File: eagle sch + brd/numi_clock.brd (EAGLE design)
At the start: 100 x 80 mm, 35 parts, among them IC1 MEGA8-AI, IC2 LM75, Q1 12MHz, Y1 32.768kHz

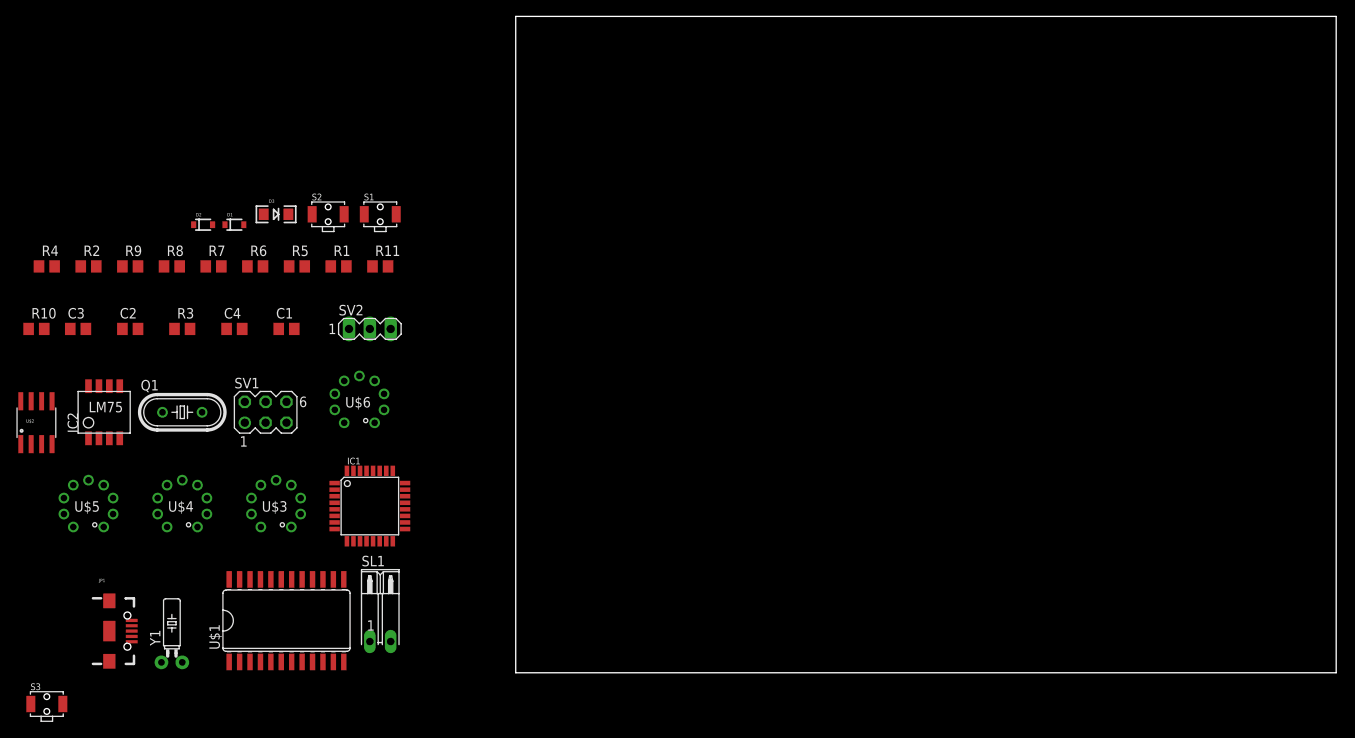
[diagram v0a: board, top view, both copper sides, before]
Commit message: minor changes
minor changes
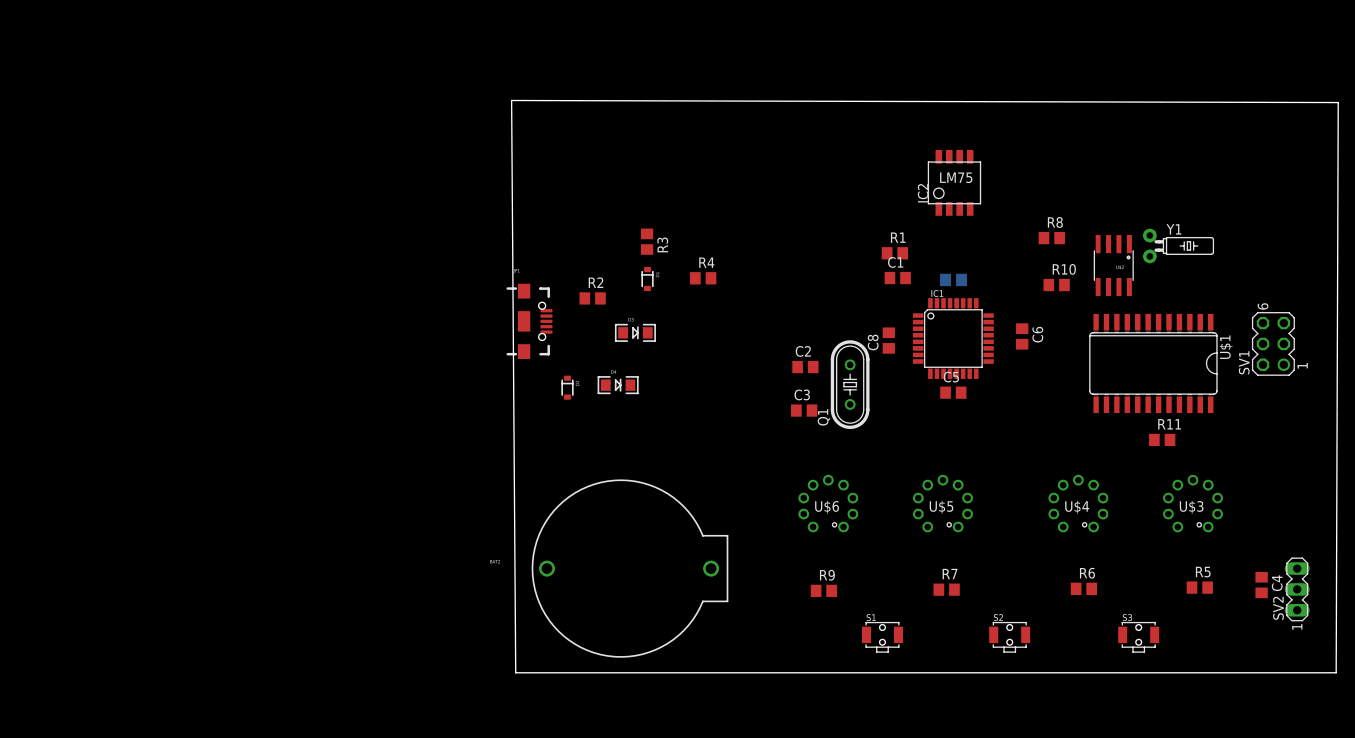
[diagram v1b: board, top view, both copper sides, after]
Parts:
- removed SL1: VBATT, con-amp-quick:02PA
- added BAT2: cr2032, SparkFun:BATTCOM_20MM_PTH
- added C5, C6, C7, C8: 100nF, rcl:C0805
- added D4: red, SparkFun-LED:LED-1206
- moved S3 133.3 mm to (75.9, 4.62)
- moved U$2 132.7 mm to (72.9, 49.6), turned to 180 degrees
- moved Y1 129.6 mm to (77.3, 52.0), turned to 270 degrees
- moved C4 129.0 mm to (90.9, 10.7), turned to 270 degrees
- moved R10 124.5 mm to (65.9, 47.3)
- moved SV1 123.1 mm to (92.3, 40.1), turned to 90 degrees
- moved SV2 117.4 mm to (95.2, 10.2), turned to 90 degrees
- moved R5 116.8 mm to (83.4, 10.4)
- moved U$3 111.8 mm to (82.5, 20.3)
- moved U$1 110.2 mm to (77.7, 37.7), turned to 180 degrees
- moved U$4 109.2 mm to (68.6, 20.3)
- moved R6 108.4 mm to (69.2, 10.2)
- moved IC2 107.3 mm to (52.8, 59.7)
- moved R8 107.3 mm to (65.3, 53.0)
- moved U$5 104.1 mm to (52.1, 20.3)
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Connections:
- removed net +3V3: R5.1, R6.1, R7.1, R9.1, SL1.2, U$2.3
- new net LED: D4.A, IC1.22
- new net N$6: BAT2.1, U$2.3
- net +5V: now also C5.2, C6.2, C7.2, C8.2, R5.1, R6.1, R7.1, R9.1
- net GND: now also BAT2.2, C5.1, C6.1, C7.1, C8.1, D4.C; no longer SL1.1
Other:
- board size 100 x 80 mm -> 100.8 x 69.8 mm

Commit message: layout adjustments
layout adjustments
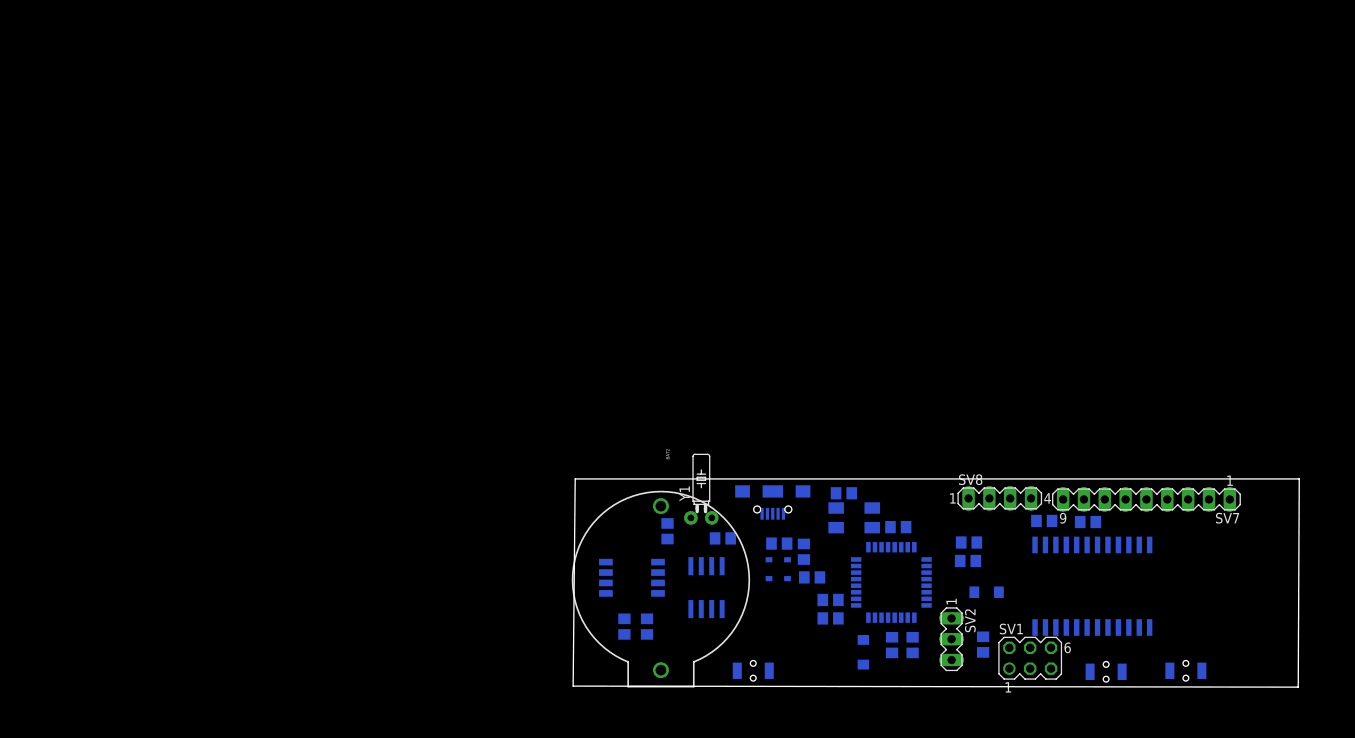
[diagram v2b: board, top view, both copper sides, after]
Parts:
- removed R5, R6, R7: 10k, rcl:R0805
- removed U$3, U$4, U$5, U$6: IV-9, domestichacks:IV-9
- added C10, C9: 27pF, rcl:C0805
- added SV7: dig0, con-lstb:MA09-1
- added SV8: conn digits, con-lstb:MA04-1
- C2, C3: value 27pF -> 22pF
- Q1: device crystal:HC49/S -> crystal:CTS406
- moved R8 70.4 mm to (13.2, 5.62), flipped to the bottom, turned to 270 degrees
- moved R10 65.0 mm to (16.0, 5.62), flipped to the bottom, turned to 270 degrees
- moved Y1 63.9 mm to (22.6, 18.9), turned to 0 degrees
- moved U$2 63.3 mm to (23.2, 10.4), flipped to the bottom
- moved IC2 61.2 mm to (14.2, 12.2), flipped to the bottom, turned to 270 degrees
- moved D4 51.5 mm to (57.4, 9.81), flipped to the bottom, turned to 180 degrees
- moved SV1 48.4 mm to (62.7, 1.77), turned to 0 degrees
- moved D3 47.8 mm to (42.4, 2.50), flipped to the bottom, turned to 270 degrees
- moved R1 47.8 mm to (45.9, 3.38), flipped to the bottom, turned to 270 degrees
- moved R3 45.6 mm to (36.1, 11.6), flipped to the bottom, turned to 0 degrees
- moved C1 44.8 mm to (48.4, 3.38), flipped to the bottom, turned to 90 degrees
- moved SV2 42.6 mm to (53.1, 4.09), turned to 270 degrees
- moved R2 40.2 mm to (35.1, 14.8), flipped to the bottom, turned to 90 degrees
- moved C6 39.7 mm to (38.4, 8.88), flipped to the bottom, turned to 180 degrees
- moved D1 39.3 mm to (33.1, 12.6), flipped to the bottom
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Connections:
- net +5V: no longer R5.1, R6.1, R7.1
- net A: now also SV7.5; no longer U$3.5, U$4.5, U$5.5, U$6.5
- net B: now also SV7.3; no longer U$3.3, U$4.3, U$5.3, U$6.3
- net C: now also SV7.4; no longer U$3.4, U$4.4, U$5.4, U$6.4
- net D: now also SV7.8; no longer U$3.8, U$4.8, U$5.8, U$6.8
- net DIG0: now also SV7.1, SV8.1; no longer U$6.1
- net DIG1: now also SV8.2; no longer R7.2, U$5.1
- net DIG2: now also SV8.3; no longer R6.2, U$4.1
- net DIG3: now also SV8.4; no longer R5.2, U$3.1
- net DP: now also SV7.2; no longer U$3.2, U$4.2, U$5.2, U$6.2
- net E: now also SV7.9; no longer U$3.9, U$4.9, U$5.9, U$6.9
- net F: now also SV7.6; no longer U$3.6, U$4.6, U$5.6, U$6.6
- net G: now also SV7.7; no longer U$3.7, U$4.7, U$5.7, U$6.7
- net GND: now also C10.1, C9.1; no longer JP1.ID1
- net N$1: now also Q1.3; no longer Q1.2
- net N$4: now also C9.2, Y1.1; no longer Y1.2
- net N$5: now also C10.2, Y1.2; no longer Y1.1
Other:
- board size 100.8 x 69.8 mm -> 88.5 x 25.4 mm

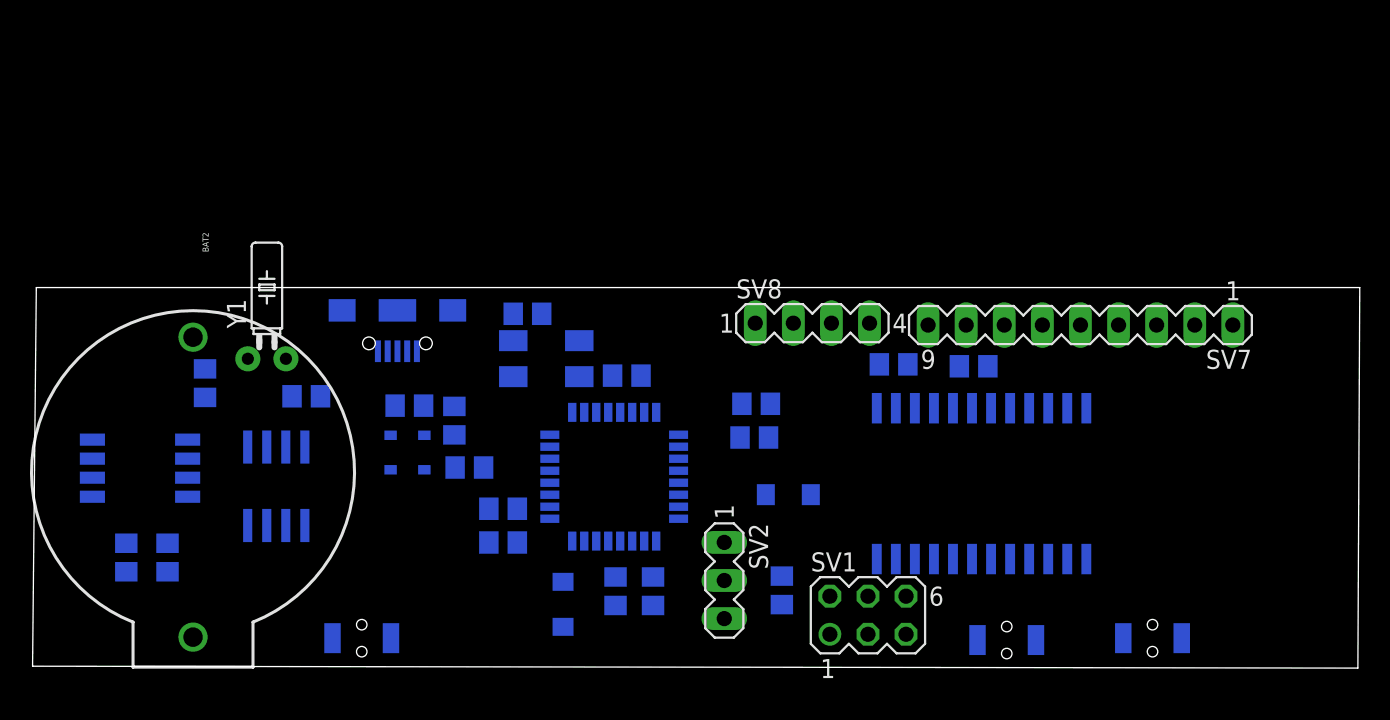
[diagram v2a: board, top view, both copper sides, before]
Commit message: layout adjustments
layout adjustments
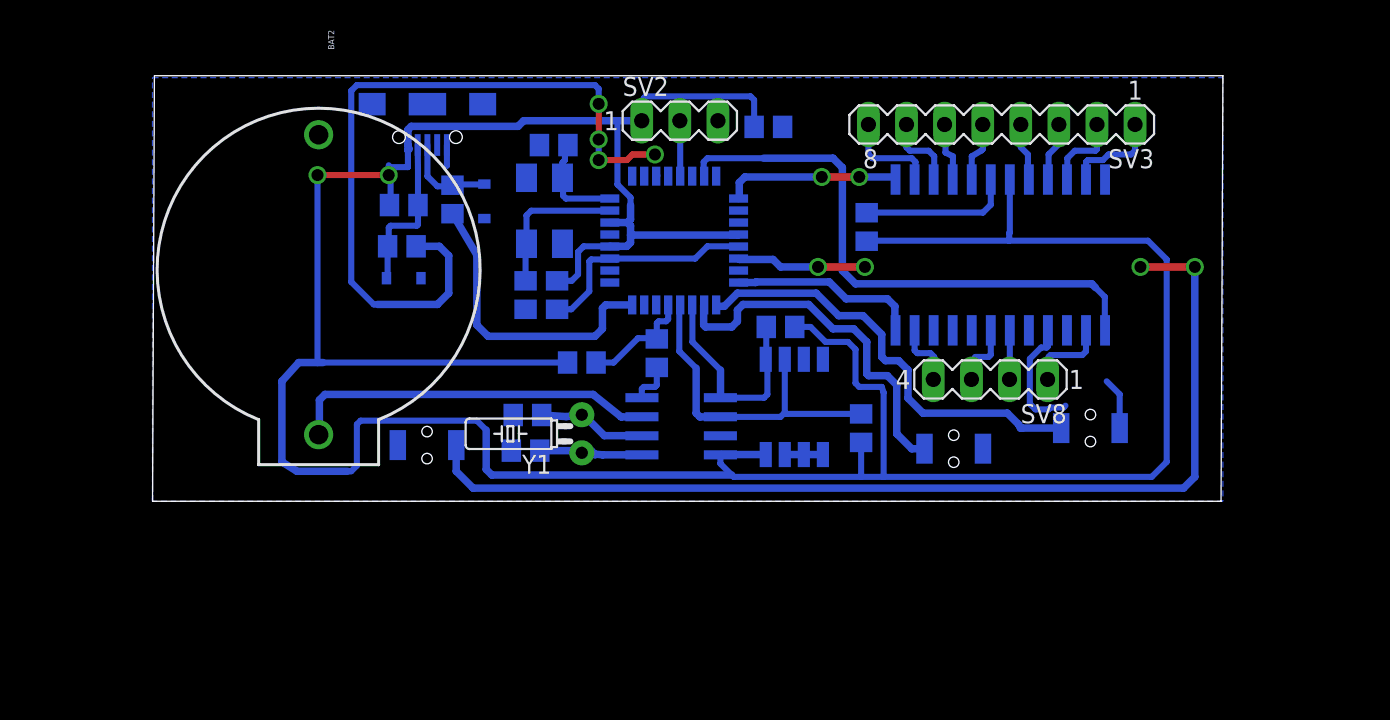
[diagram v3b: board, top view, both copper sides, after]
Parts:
- removed C6, C7, C8: 100nF, rcl:C0805
- removed D3, D4: red, SparkFun-LED:LED-1206
- removed R9: 10k, rcl:R0805
- removed SV1: SPI, con-lstb:MA03-2
- removed SV7: dig0, con-lstb:MA09-1
- added SV3: (no value), con-lstb:MA08-1
- moved S3 50.1 mm to (33.3, 13.1)
- moved R10 47.0 mm to (62.2, 14.2), turned to 90 degrees
- moved R8 46.3 mm to (56.9, 21.0), turned to 0 degrees
- moved IC2 43.1 mm to (57.2, 15.7), turned to 180 degrees
- moved S1 41.4 mm to (68.4, 12.9), turned to 180 degrees
- moved C4 30.9 mm to (56.1, 34.3), turned to 0 degrees
- moved SV2 30.8 mm to (50.2, 34.8), turned to 0 degrees
- moved U$2 27.3 mm to (50.2, 14.4), turned to 90 degrees
- moved C9 21.8 mm to (39.9, 12.8), turned to 180 degrees
- moved Y1 21.6 mm to (43.6, 13.9), turned to 90 degrees
- moved R3 18.0 mm to (31.8, 29.1), turned to 180 degrees
- moved D2 17.9 mm to (37.1, 29.4)
- moved C5 16.9 mm to (42.0, 23.1), turned to 90 degrees
- moved IC1 16.2 mm to (49.8, 26.8)
- moved BAT2 15.9 mm to (26.1, 33.8)
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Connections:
- removed net LED: D4.A, IC1.22
- removed net MISO: IC1.16, SV1.1
- new net AVCC: IC1.18
- net +5V: no longer C6.2, C7.2, C8.2, D3.A, IC1.18, R9.1, SV1.2
- net A: now also SV3.8; no longer SV7.5
- net B: now also SV3.7, U$1.15; no longer SV7.3, U$1.16
- net C: now also SV3.6, U$1.16; no longer SV7.4, U$1.20
- net D: now also SV3.5, U$1.17; no longer SV7.8, U$1.23
- net DIG0: no longer R9.2, SV7.1
- net DIG1: now also U$1.6; no longer U$1.11
- net DIG2: now also U$1.7; no longer U$1.6
- net DIG3: now also U$1.11; no longer U$1.7
- net DP: now also SV3.1, U$1.23; no longer SV7.2, U$1.22
- net E: now also SV3.4, U$1.20; no longer SV7.9, U$1.21
- net F: now also SV3.3, U$1.21; no longer SV7.6, U$1.15
- net FUNC: now also IC1.22; no longer IC1.19
- net G: now also SV3.2, U$1.22; no longer SV7.7, U$1.17
- net GND: no longer C6.1, C7.1, C8.1, D3.C, D4.C, SV1.6
- net HC: now also IC1.13; no longer IC1.23
- net HOUR: now also IC1.26; no longer IC1.25
- net MINUTE: now also IC1.25; no longer IC1.26
- net MOSI: no longer SV1.4
- net N$10: now also IC1.11; no longer IC1.1
- net RESET: no longer SV1.5
- net SCK: no longer SV1.3
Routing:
- net +5V: track 0.00 -> 226.0 mm, vias 0 -> 2
- net FUNC: track 0.00 -> 77.9 mm, vias 0 -> 3
- net N$10: track 0.00 -> 50.6 mm, vias 0 -> 4
- net MOSI: track 0.00 -> 37.9 mm
- net GND: track 0.00 -> 34.1 mm
- net MINUTE: track 0.00 -> 29.2 mm
- net N$6: track 0.00 -> 24.5 mm
- net HOUR: track 0.00 -> 24.3 mm
- net SCL: track 0.00 -> 22.5 mm
- net N$9: track 0.00 -> 20.2 mm
- net SDA: track 0.00 -> 14.8 mm
- net CS: track 0.00 -> 12.8 mm
- net SCK: track 0.00 -> 11.9 mm, vias 0 -> 2
- net N$8: track 0.00 -> 10.8 mm
- net N$3: track 0.00 -> 10.2 mm
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- added copper zone on layer 16, net GND
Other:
- board size 88.5 x 25.4 mm -> 71.4 x 28.4 mm

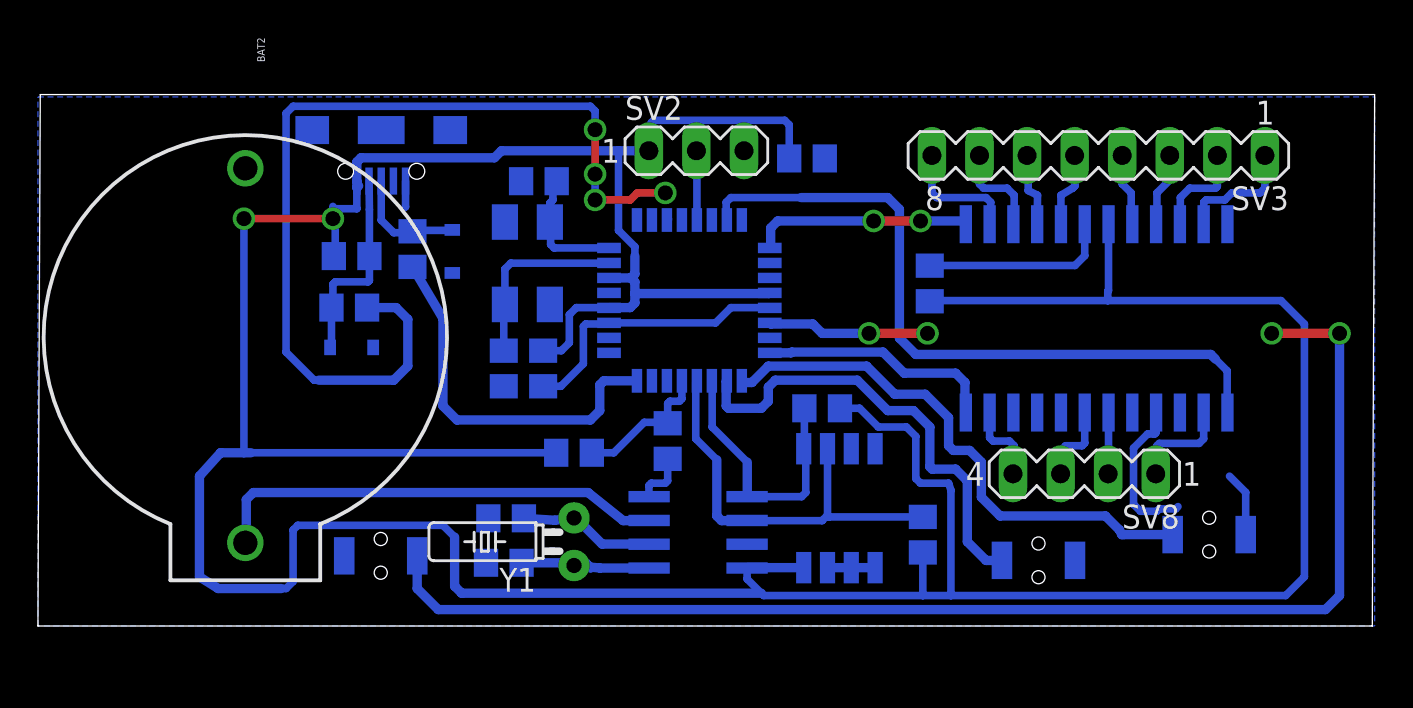
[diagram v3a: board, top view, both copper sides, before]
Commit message: later edit
later edit
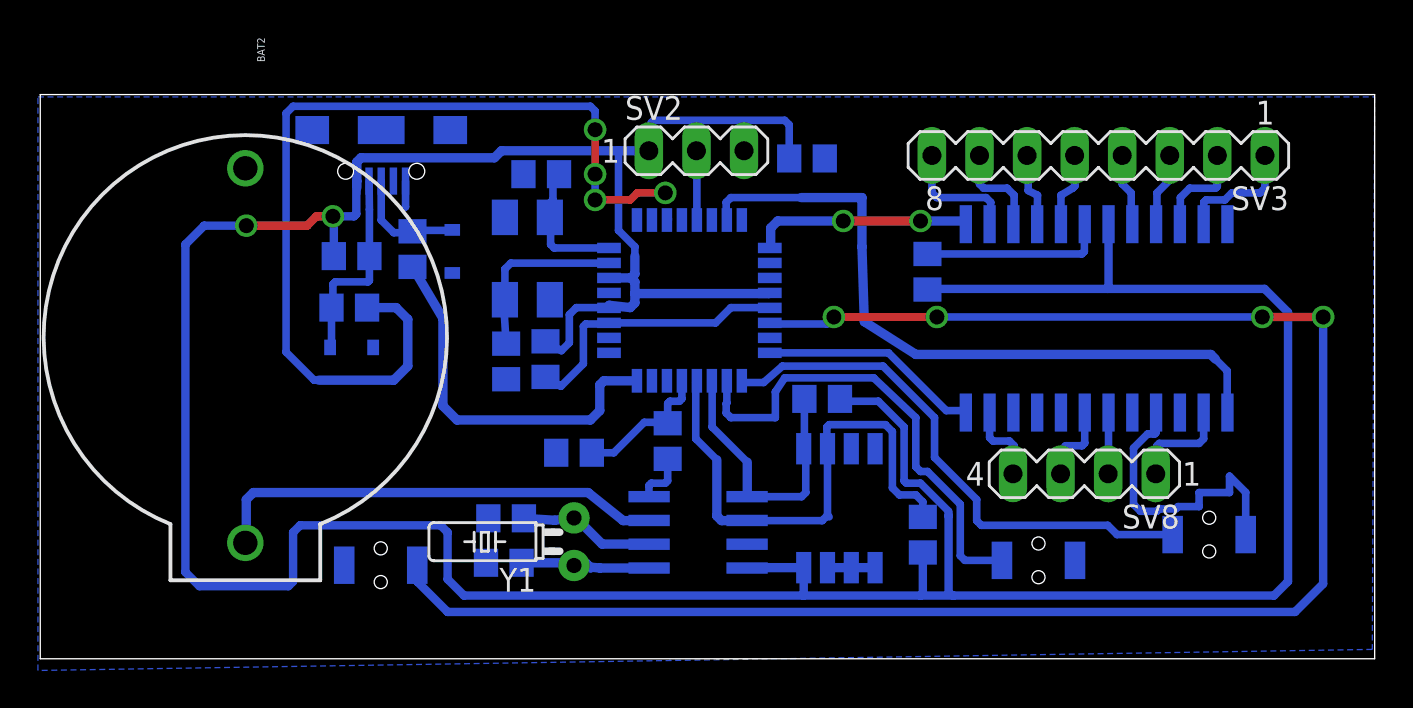
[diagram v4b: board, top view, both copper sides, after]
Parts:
- moved R11 0.64 mm to (62.5, 28.3)
- moved C5 0.52 mm to (42.1, 23.6)
- moved R8 0.50 mm to (56.9, 21.5)
- moved S3 0.50 mm to (33.3, 12.6)
- moved C2 0.40 mm to (40.0, 23.5)
- moved C3 0.40 mm to (41.9, 33.5)
- moved Q1 0.25 mm to (41.1, 29.0)
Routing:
- net +5V: track 226.0 -> 208.1 mm
- net FUNC: track 77.9 -> 94.5 mm, vias 3 -> 4
- net SCL: track 22.5 -> 28.1 mm
- net GND: track 34.1 -> 38.7 mm
- net HOUR: track 24.3 -> 25.5 mm
- net CS: track 12.8 -> 11.9 mm
- net SDA: track 14.8 -> 15.3 mm
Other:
- board size 71.4 x 28.4 mm -> 71.2 x 30.1 mm
